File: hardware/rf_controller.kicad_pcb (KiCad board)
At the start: 2 copper layers, 62 x 52 mm, 32 parts, among them SW1 SWITCH, SW2 BUTTON, SW3 BUTTON, SW4 BUTTON, U1 ENC_E11X

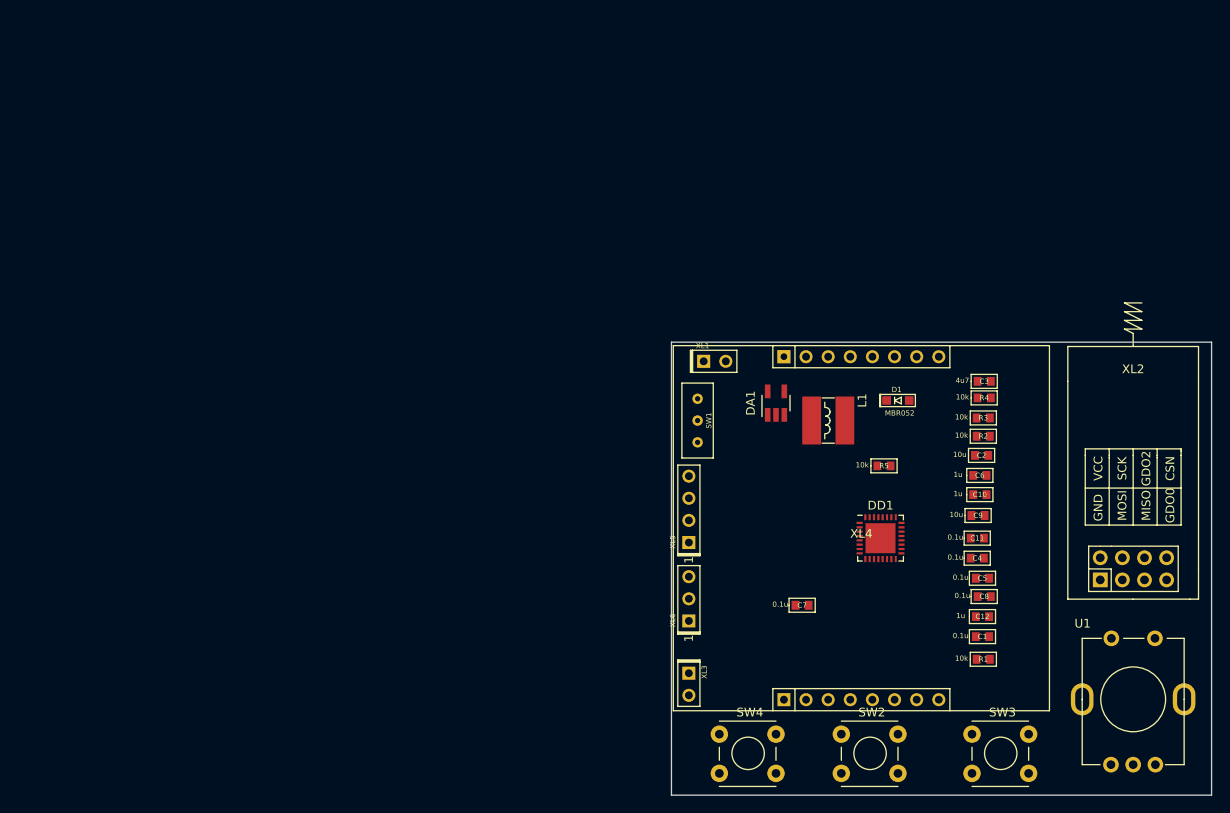
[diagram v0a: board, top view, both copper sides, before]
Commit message: + Add FW project; + Add HW gerber files.
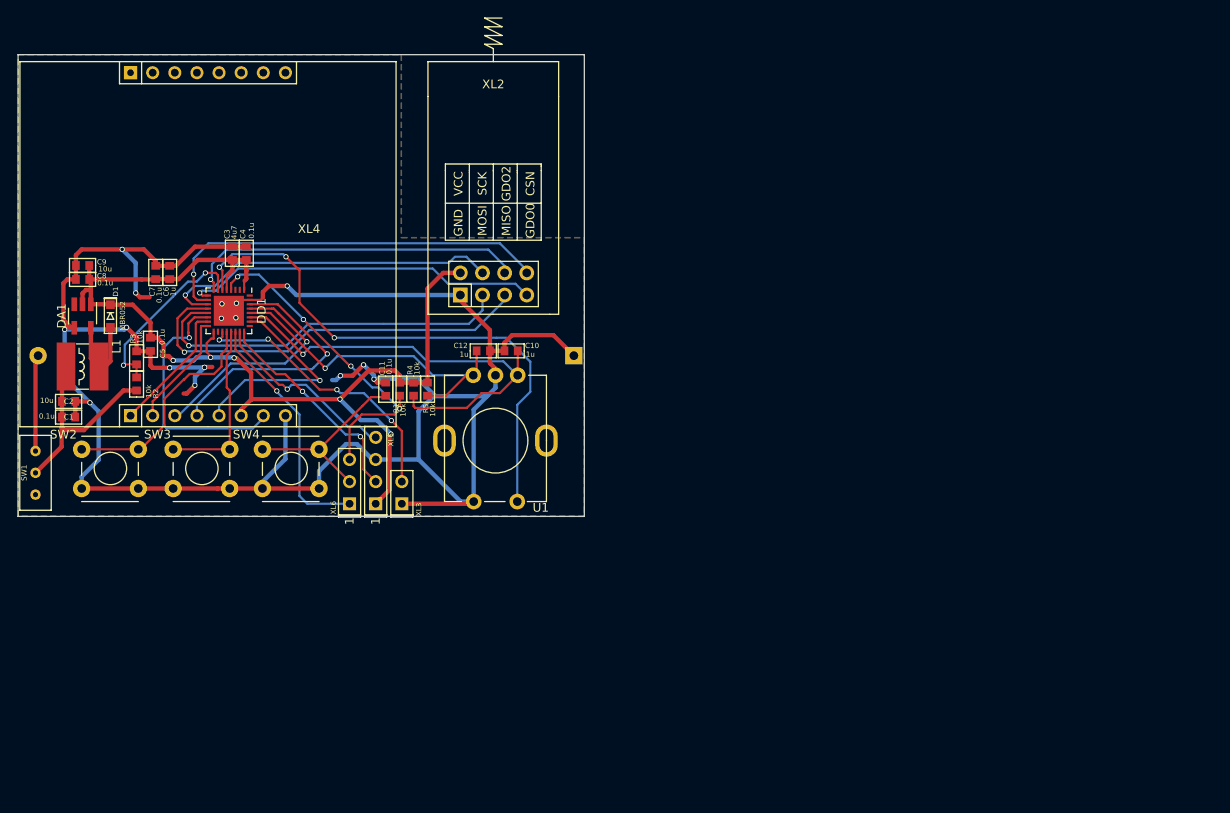
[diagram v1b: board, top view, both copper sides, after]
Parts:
- R1, R2, R3, R4, R5: footprint Capacitors:CAP_0603 -> Resistors:RES_0603
- SW2: value BUTTON -> BUTTON1
- SW3: value BUTTON -> BUTTON2
- SW4: value BUTTON -> BUTTON3/RST
- XL1: footprint Connectors:PLS-2 -> Installation:2xBAT_AA_SOLDER; moved to B.Cu
- moved C8 109.7 mm to (60.4, 62.8), turned to 180 degrees
- moved C1 107.9 mm to (58.8, 78.6)
- moved C9 106.7 mm to (60.4, 61.2), turned to 180 degrees
- moved C2 105.0 mm to (58.8, 76.8)
- moved C5 99.2 mm to (68.2, 70.2), turned to 270 degrees
- moved R3 97.4 mm to (66.6, 71.8), turned to 90 degrees
- moved R2 97.4 mm to (66.6, 74.8), turned to 90 degrees
- moved SW3 97.4 mm to (70.3, 87.3)
- moved C6 95.9 mm to (70.4, 62.0), turned to 90 degrees
- moved SW2 93.1 mm to (59.8, 87.3)
- moved D1 90.9 mm to (63.6, 67.0), turned to 270 degrees
- moved C4 90.9 mm to (79.2, 59.8), turned to 90 degrees
- moved C3 87.5 mm to (77.6, 59.8), turned to 90 degrees
- moved L1 85.8 mm to (60.4, 72.8)
- moved C7 83.5 mm to (68.8, 62.0), turned to 90 degrees
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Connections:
- net Net-(D1-PadA) renamed /PWR_IN
- net Net-(SW1-Pad1) renamed /BAT
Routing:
- net GND: track 0.00 -> 270.0 mm, vias 0 -> 17
- net +3.3V: track 0.00 -> 120.2 mm, vias 0 -> 5
- net /BUTTON0: track 0.00 -> 63.0 mm, vias 0 -> 3
- net /ENCODER_CH1: track 0.00 -> 51.8 mm, vias 0 -> 1
- net /CC1101_CS: track 0.00 -> 48.1 mm, vias 0 -> 1
- net /CC1101_MISO: track 0.00 -> 48.0 mm, vias 0 -> 1
- net /CC1101_MOSI: track 0.00 -> 44.1 mm, vias 0 -> 1
- net /CC1101_GDO0: track 0.00 -> 41.5 mm, vias 0 -> 1
- net /CC1101_CLK: track 0.00 -> 40.3 mm, vias 0 -> 1
- net /CC1101_GDO2: track 0.00 -> 40.2 mm, vias 0 -> 1
- net /RST: track 0.00 -> 39.3 mm, vias 0 -> 4
- net /ENCODER_CH2: track 0.00 -> 39.0 mm, vias 0 -> 1
- net /DBG_TX: track 0.00 -> 32.4 mm, vias 0 -> 4
- net /LCD_DIN: track 0.00 -> 30.0 mm, vias 0 -> 1
- net /LCD_BCKLT: track 0.00 -> 29.2 mm, vias 0 -> 1
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- added copper zone on B.Cu, net GND
- added copper zone on F.Cu, net GND
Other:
- board size 62 x 52 mm -> 65 x 53 mm
- net class PWR added: clearance 0.2, trace_width 0.5, via_dia 0.6, via_drill 0.4
- board text added: "RF controller, v.0.1 @RJ"
